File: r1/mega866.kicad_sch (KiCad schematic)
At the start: 40 parts, among them J1 ZSM1-SM1, J10 Conn_01x06_Male, J12 tl866_dip40, J13 tl866_dip40, J2 ZSM1-SM2, J3 tl866_dip40, J4 tl866_dip40, J5 Conn_01x02_Male, J6 Conn_01x06_Male, J7 Conn_01x06_Male, J8 Conn_01x02_Male, J9 Conn_01x06_Male, Q1 BSS84, Q2 2N7002, Q3 2N7002, U1 Pico

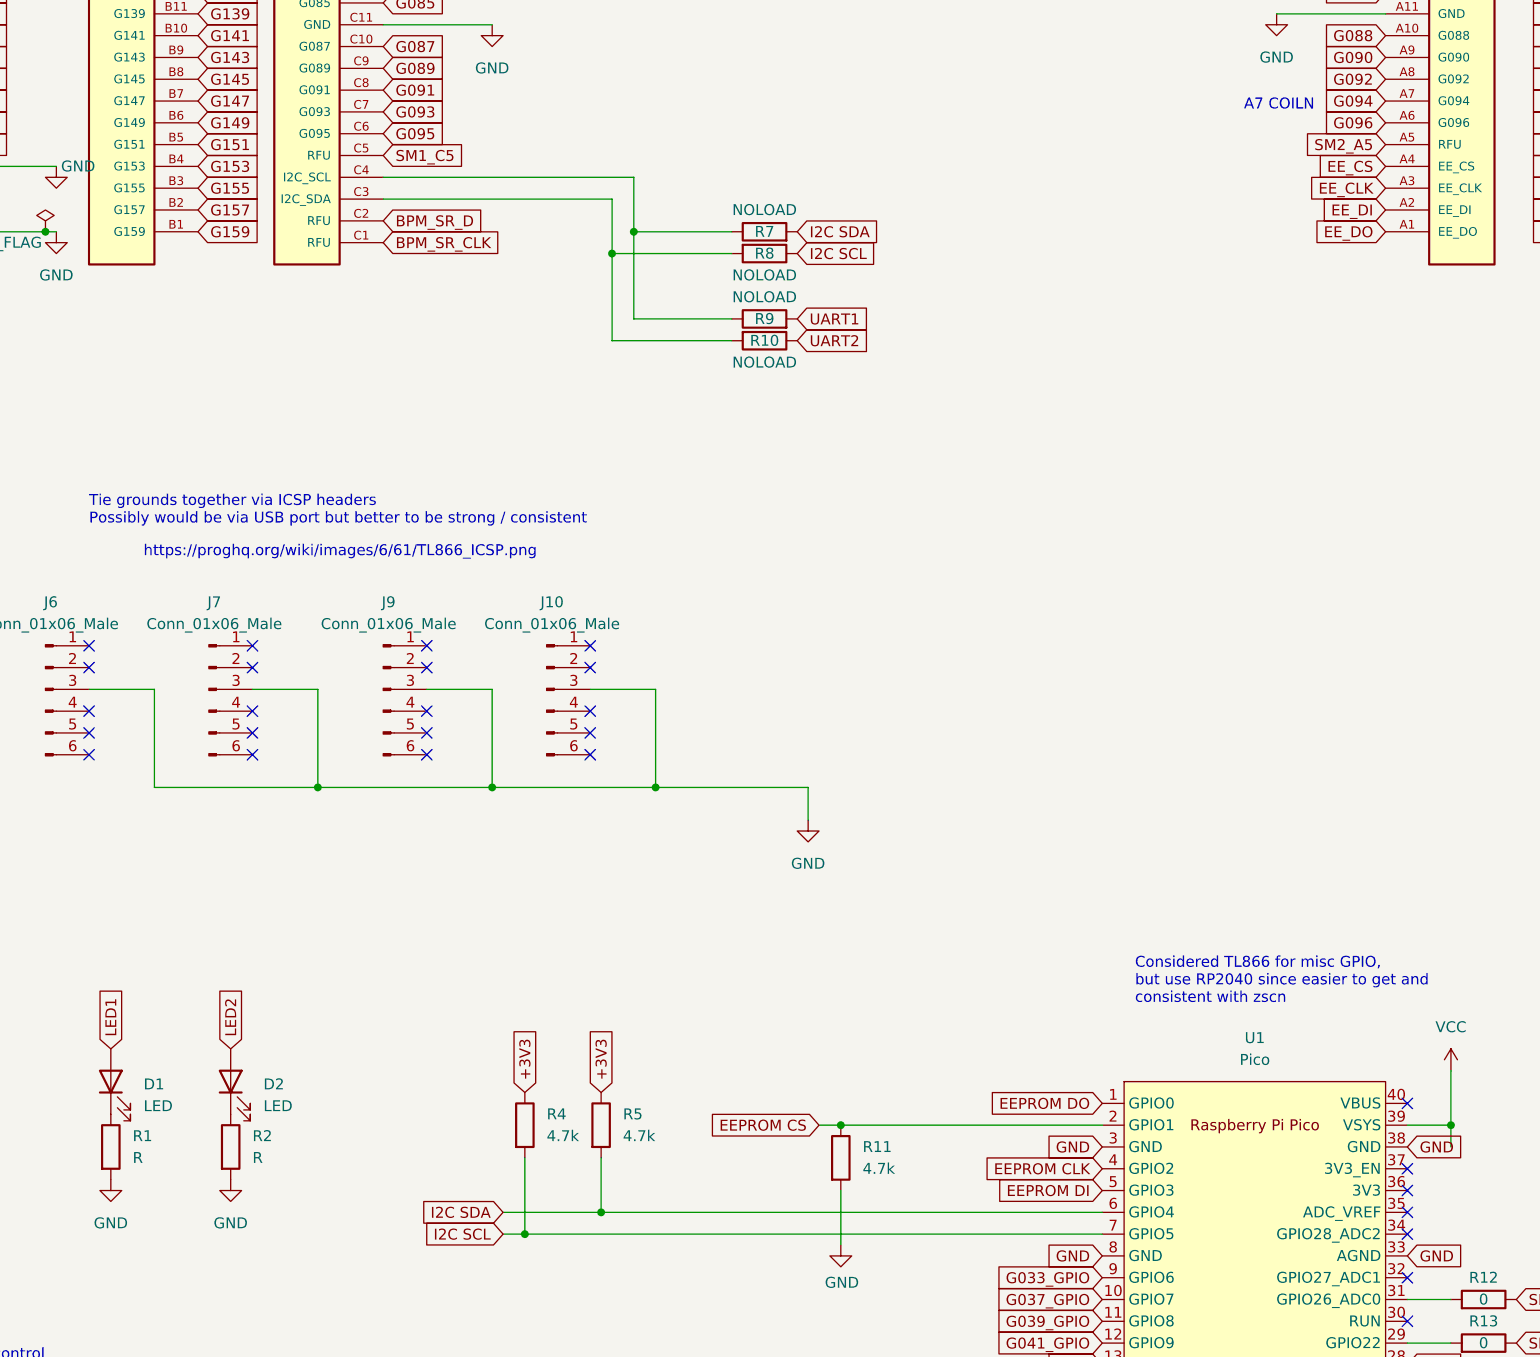
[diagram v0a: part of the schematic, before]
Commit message: cleaner drc / fix errors
Signed-off-by: John McMaster <johndmcmaster@gmail.com>
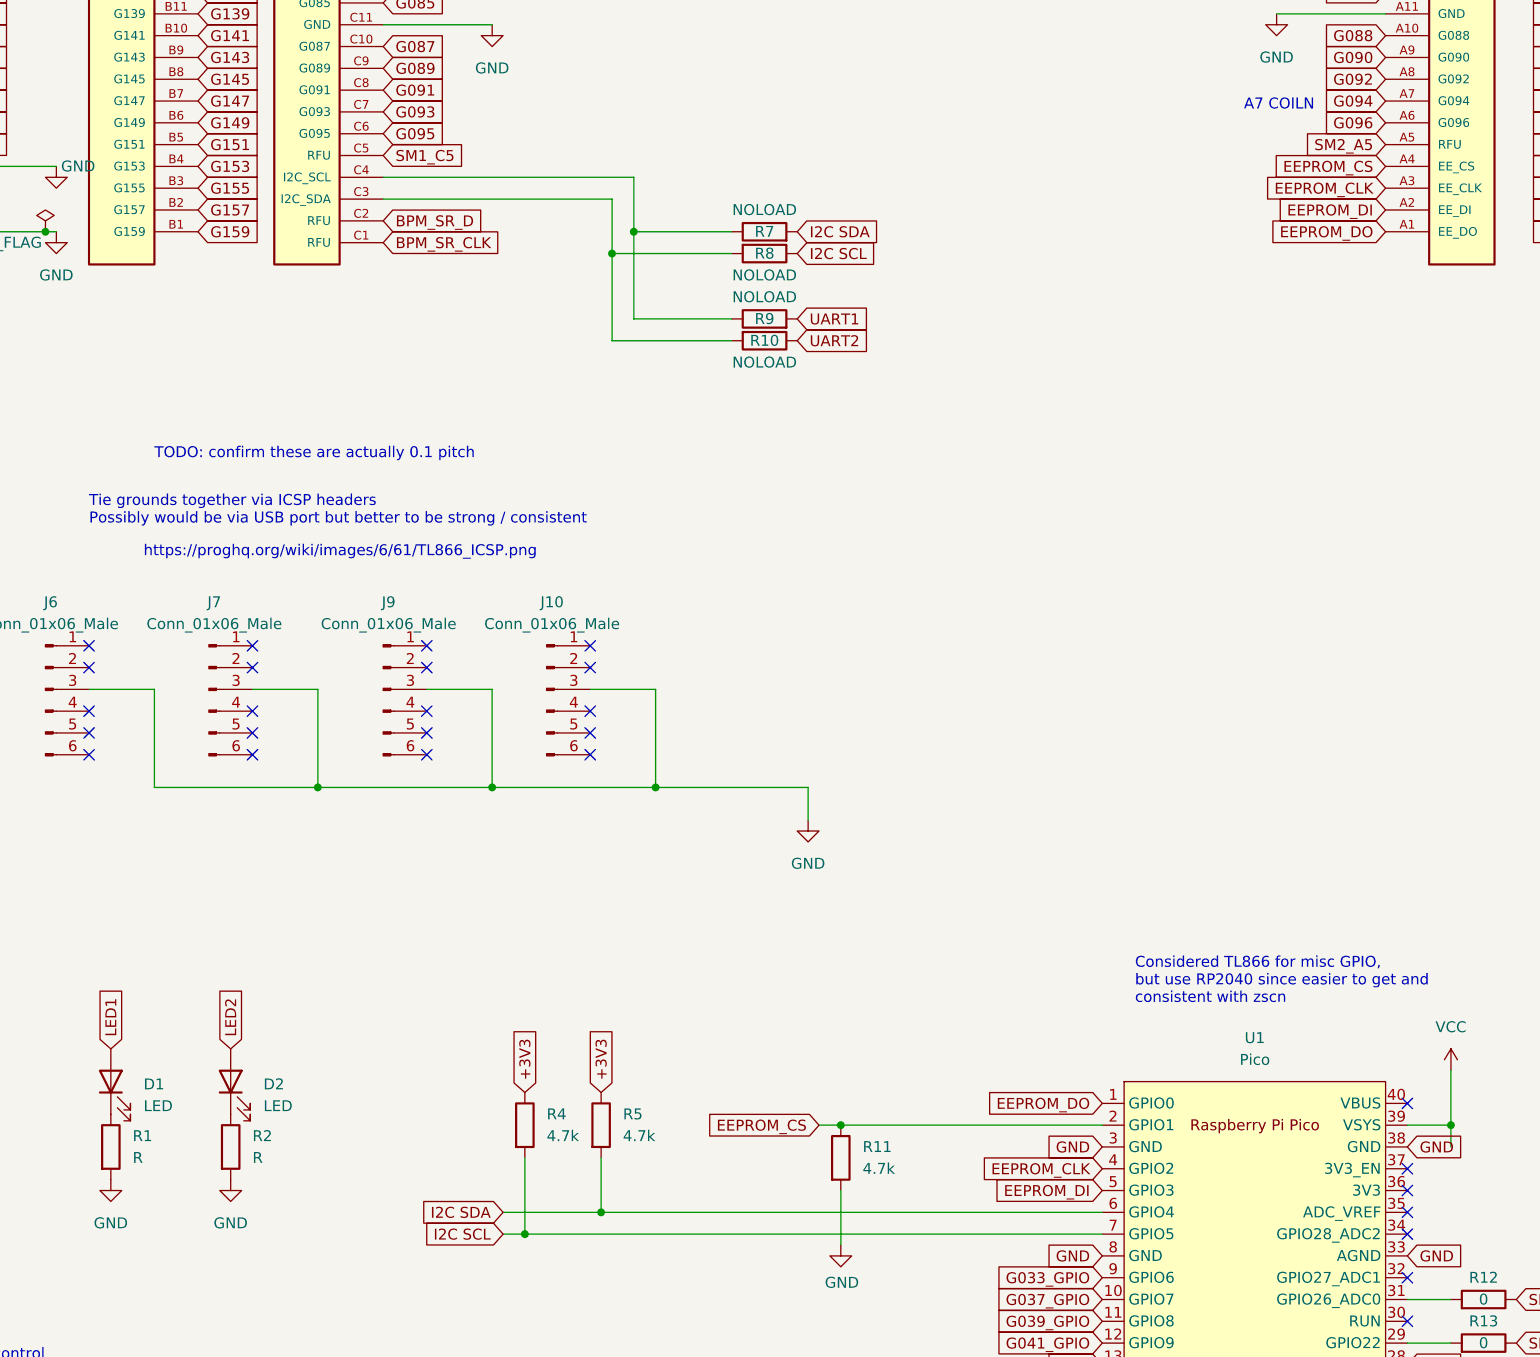
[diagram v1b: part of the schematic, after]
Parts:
- D1, D2: footprint (none) -> LED_SMD:LED_0603_1608Metric
- J1: footprint zsm:5650470-5 -> TE_5650933-5; symbol zsm:ZSM1-SM1 -> mega866:ZSM1-SM1
- J10, J6, J7, J9: footprint (none) -> Connector_PinHeader_2.54mm:PinHeader_1x06_P2.54mm_Vertical
- J2: symbol zsm:ZSM1-SM2 -> mega866:ZSM1-SM2
- J5, J8: footprint (none) -> Connector_PinHeader_2.54mm:PinHeader_1x02_P2.54mm_Vertical
- R1, R2: footprint (none) -> Resistor_SMD:R_0603_1608Metric
- U1: footprint MCU_RaspberryPi_and_Boards:RPi_Pico_SMD_TH -> mega866:RPi_Pico_SMD_TH; symbol MCU_RaspberryPi_and_Boards:Pico -> mega866:Pico
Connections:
- net EE_CLK is gone; now on net EEPROM_CLK: J2.A3 (EE_CLK)
- net EE_CS is gone; now on net EEPROM_CS: J2.A4 (EE_CS)
- net EE_DI is gone; now on net EEPROM_DI: J2.A2 (EE_DI)
- net EE_DO is gone; now on net EEPROM_DO: J2.A1 (EE_DO)
- net EEPROM CLK renamed EEPROM_CLK
- net EEPROM CS renamed EEPROM_CS
- net EEPROM DI renamed EEPROM_DI
- net EEPROM DO renamed EEPROM_DO
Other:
- note added: "TODO: confirm these are actually 0.1 pitch"
